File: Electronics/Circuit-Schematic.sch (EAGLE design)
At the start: 17 parts, among them IC1 7805T, U1 ARDUINOR3-BPLACE

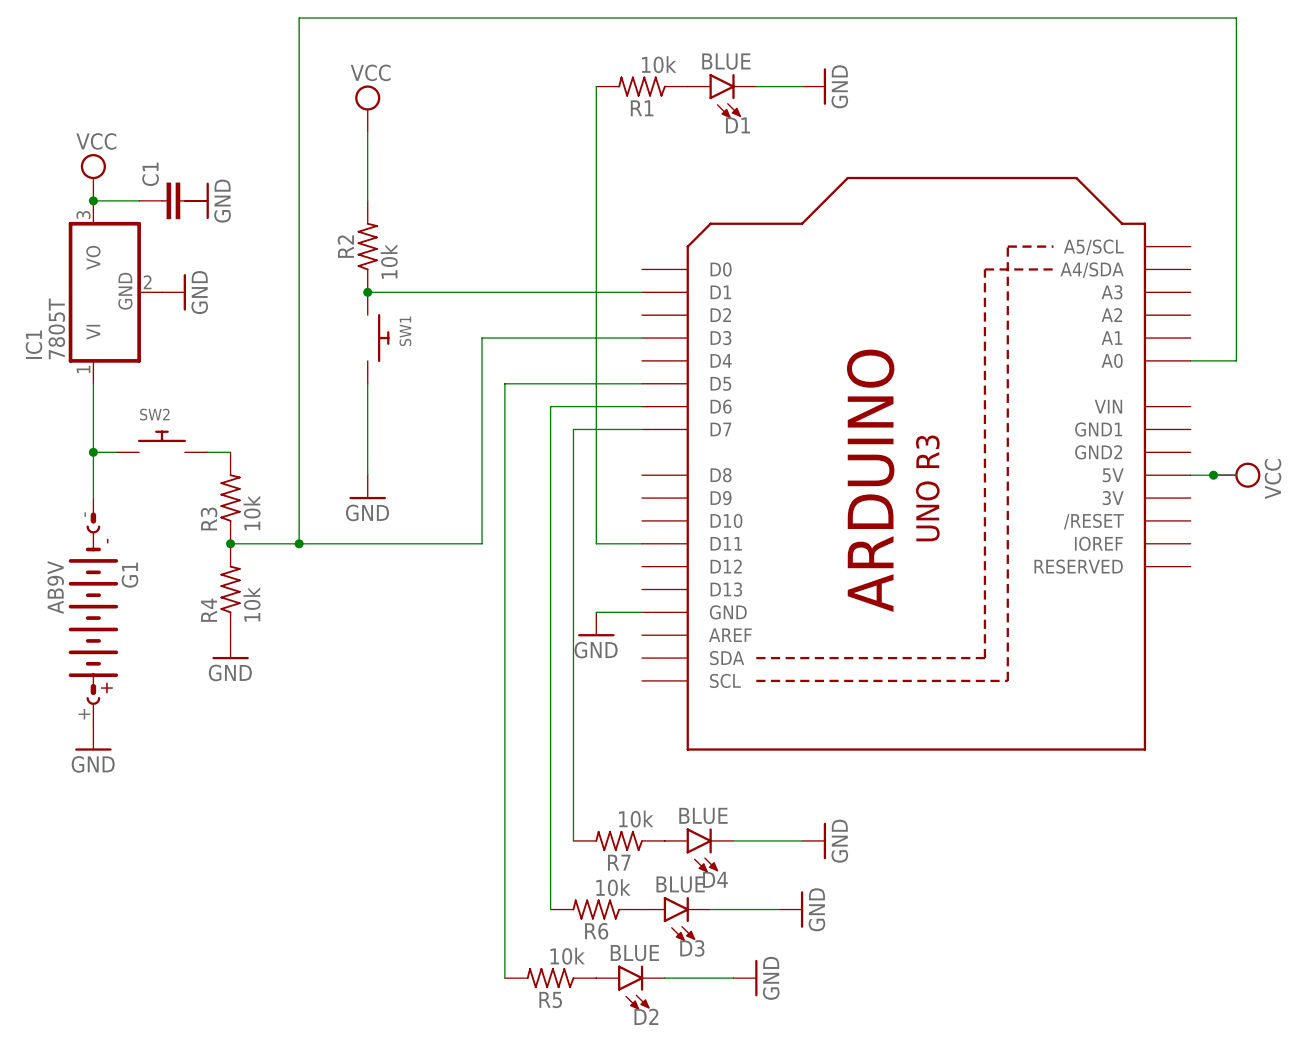
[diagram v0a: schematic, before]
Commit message: Updated all electronics files
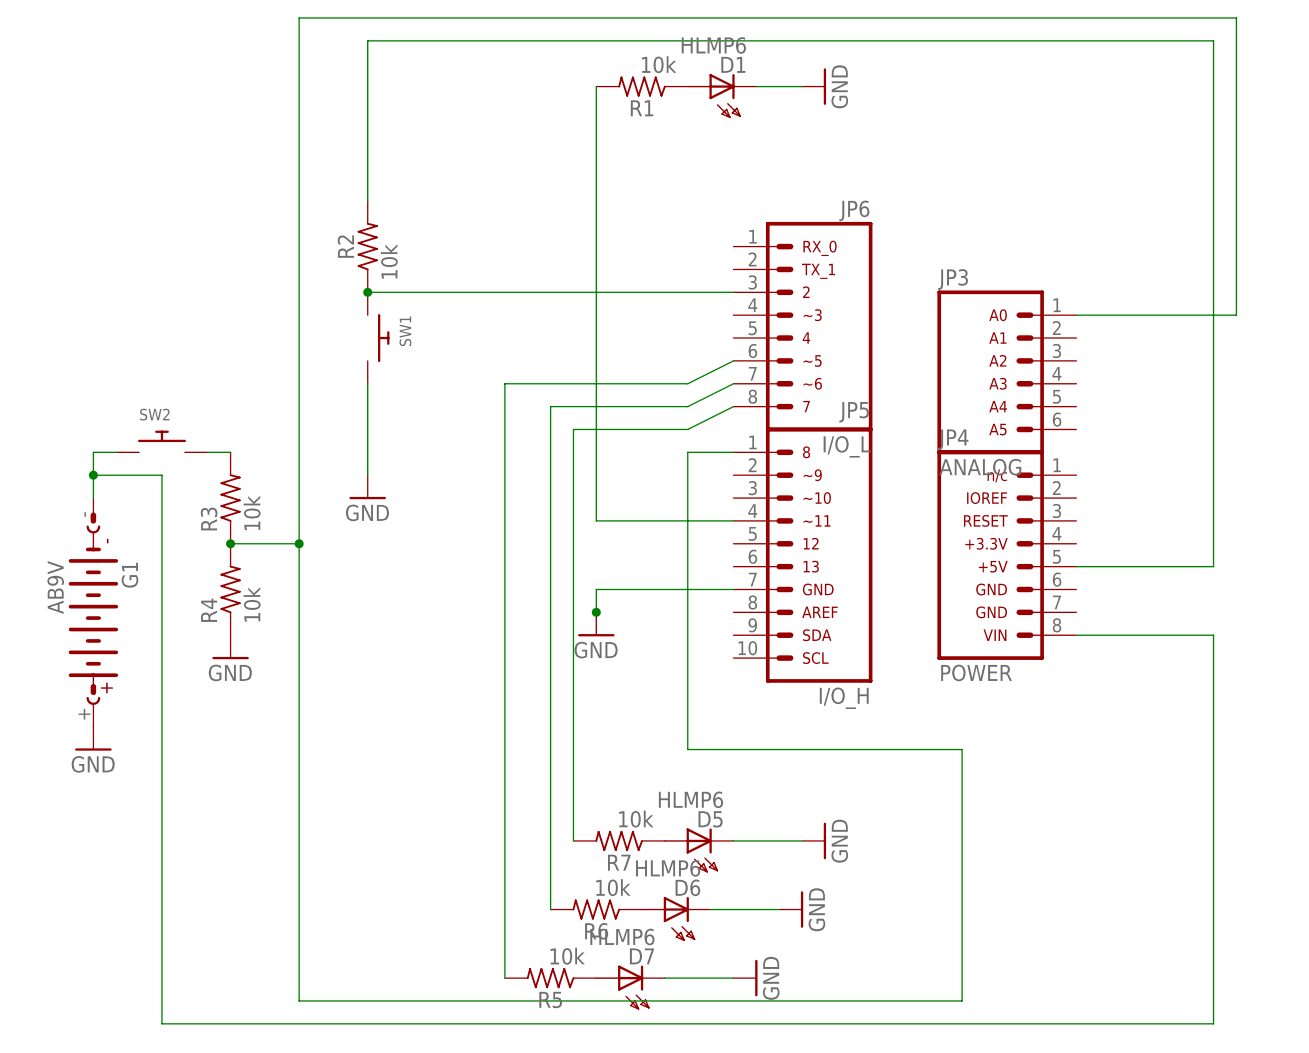
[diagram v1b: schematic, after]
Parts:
- removed C1: (no value), capacitor-wima:C10/5
- removed D2, D3, D4: BLUE, SparkFun-LED:LED-BLUE1206
- removed IC1: 7805T, adafruit:7805T
- removed U1: ARDUINOR3-BPLACE, adafruit:ARDUINOR3-BPLACE
- added D5, D6, D7: HLMP6, display-hp:HLMP6
- added JP3: (no value), arduino_jw:ARDUINO_CONN-ANALOGSIP
- added JP4: (no value), arduino_jw:ARDUINO_CONN-POWERSIP
- added JP5: ARDUINO_CONN-IO_HSIP, arduino_jw:ARDUINO_CONN-IO_HSIP
- added JP6: (no value), arduino_jw:ARDUINO_CONN-IO_LSIP
- D1: value BLUE -> HLMP6; device SparkFun-LED:LED-BLUE1206 -> display-hp:HLMP6
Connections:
- removed net N$12: D4.A, R7.1
- removed net VCC: C1.1, IC1.VO, R2.2, U1.5V
- new net N$14: JP4.5, R2.2
- new net N$4: D5.A, R7.1
- net GND: now also D1.K, D5.K, D6.K, D7.K, JP5.7; no longer D1.C, D2.C, D3.C, D4.C, IC1.GND, U1.GND
- net N$1: now also JP4.8; no longer IC1.VI
- net N$10: now also JP6.7; no longer U1.D6
- net N$11: now also JP6.8; no longer U1.D7
- net N$13: now also JP3.1, JP5.1; no longer U1.A0, U1.D3
- net N$2: now also JP5.4; no longer U1.D11
- net N$5: now also JP6.3; no longer U1.D1
- net N$7: now also D6.A, R6.1; no longer D2.A, R5.1
- net N$8: now also JP6.6; no longer U1.D5
- net N$9: now also D7.A, R5.1; no longer D3.A, R6.1
